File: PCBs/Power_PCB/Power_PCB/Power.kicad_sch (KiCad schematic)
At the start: 20 parts, among them J1 Conn_01x02, J12 Conn_01x02, J18 8PCV-02-006, J2 Conn_01x02, J3 Conn_01x02, Q1 SUD45P03-09, U2 AMS1117-3.3, U4 01000064Z, U5 TVS3300DRV

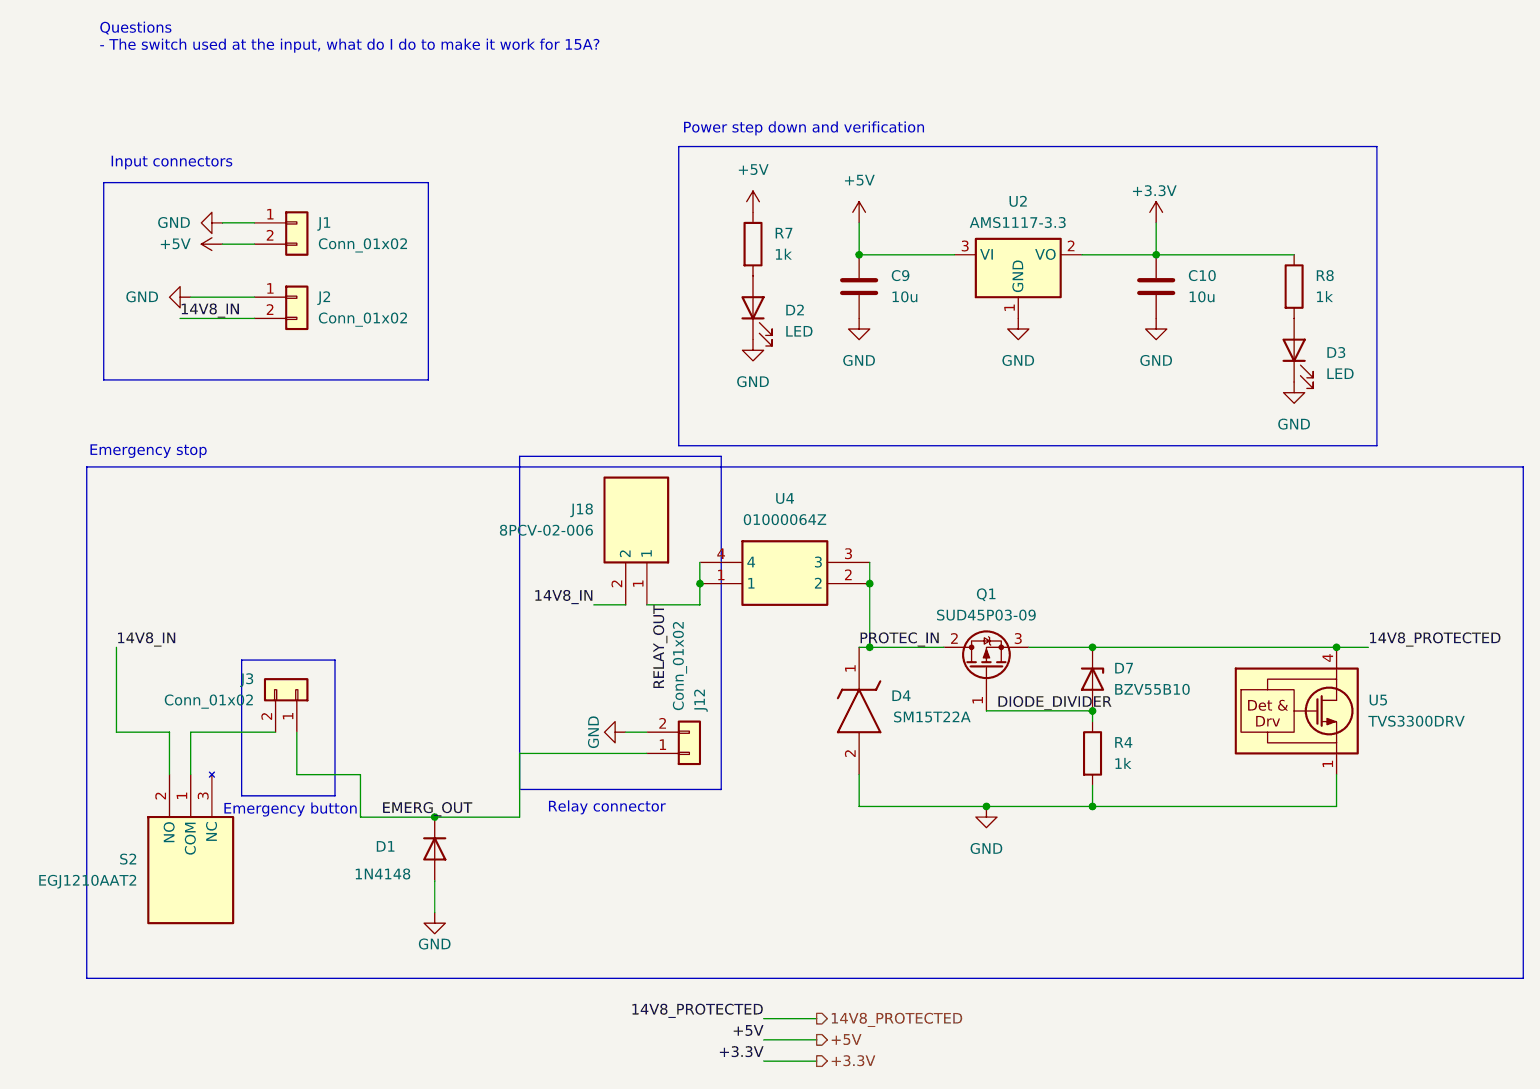
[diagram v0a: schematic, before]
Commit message: submitted power board
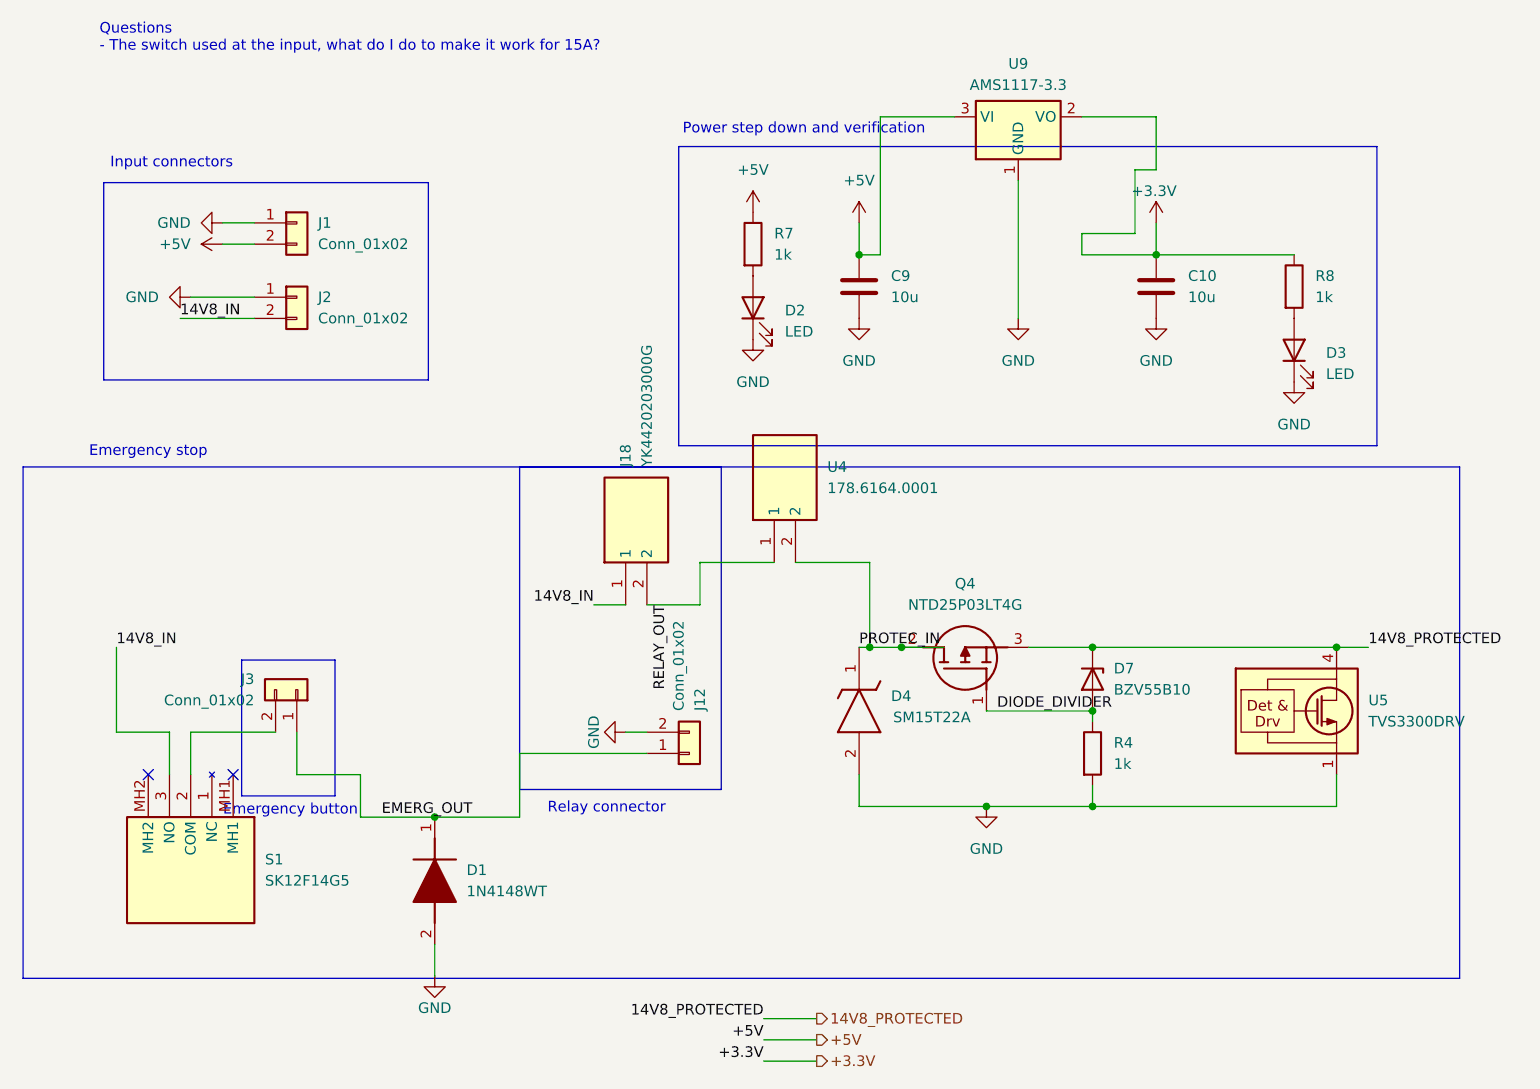
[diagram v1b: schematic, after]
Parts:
- removed D1: 1N4148, Diode_THT:D_DO-35_SOD27_P7.62mm_Horizontal, symbol Diode:1N4148
- removed J18: 8PCV-02-006, iprl_footprints:8PCV02006, symbol 8PCV-02-006:8PCV-02-006
- removed Q1: SUD45P03-09, Package_TO_SOT_SMD:TO-252-2, symbol Transistor_FET:SUD45P03-09
- removed S2: EGJ1210AAT2, iprl_footprints:EGJ1210AAT2, symbol EGJ1210AAT2:EGJ1210AAT2
- removed U2: AMS1117-3.3, Package_TO_SOT_SMD:SOT-223-3_TabPin2, symbol Regulator_Linear:AMS1117-3.3
- removed U4: 01000064Z, 01000064Z, symbol 01000064Z:01000064Z
- added D1: 1N4148WT, SODFL1608X70N, symbol 1N4148WT:1N4148WT
- added J18: YK4420203000G, RHDR2W120P0X950_1X2_2050X1430X1790P, symbol YK4420203000G:YK4420203000G
- added Q4: NTD25P03LT4G, iprl_footprints:MJD45H11T4G, symbol NTD25P03LT4G:NTD25P03LT4G
- added S1: SK12F14G5, SK12F14G5, symbol SK12F14G5:SK12F14G5
- added U4: 178.6164.0001, 178.6164.XXX1, symbol 178_6164_0001:178.6164.0001
- added U9: AMS1117-3.3, Package_TO_SOT_SMD:SOT-223-3_TabPin2, symbol Regulator_Linear:AMS1117-3.3
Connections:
- net +3.3V: now also U9.2 (VO)
- net +5V: now also U9.3 (VI)
- net 14V8_IN: now also J18.1, S1.3 (NO)
- net 14V8_PROTECTED: now also Q4.3 (S)
- net DIODE_DIVIDER: now also Q4.1 (G)
- net EMERG_OUT: now also D1.1 (K)
- net GND: now also D1.2 (A), U9.1 (GND)
- net PROTEC_IN: now also Q4.2 (D), U4.2
- net RELAY_OUT: now also J18.2, U4.1
- net at J3.2 (Pin_2): now also S1.2 (COM)
- no-connect marks 0 -> 2
